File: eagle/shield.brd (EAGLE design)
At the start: 61.9 x 55.9 mm, 14 parts

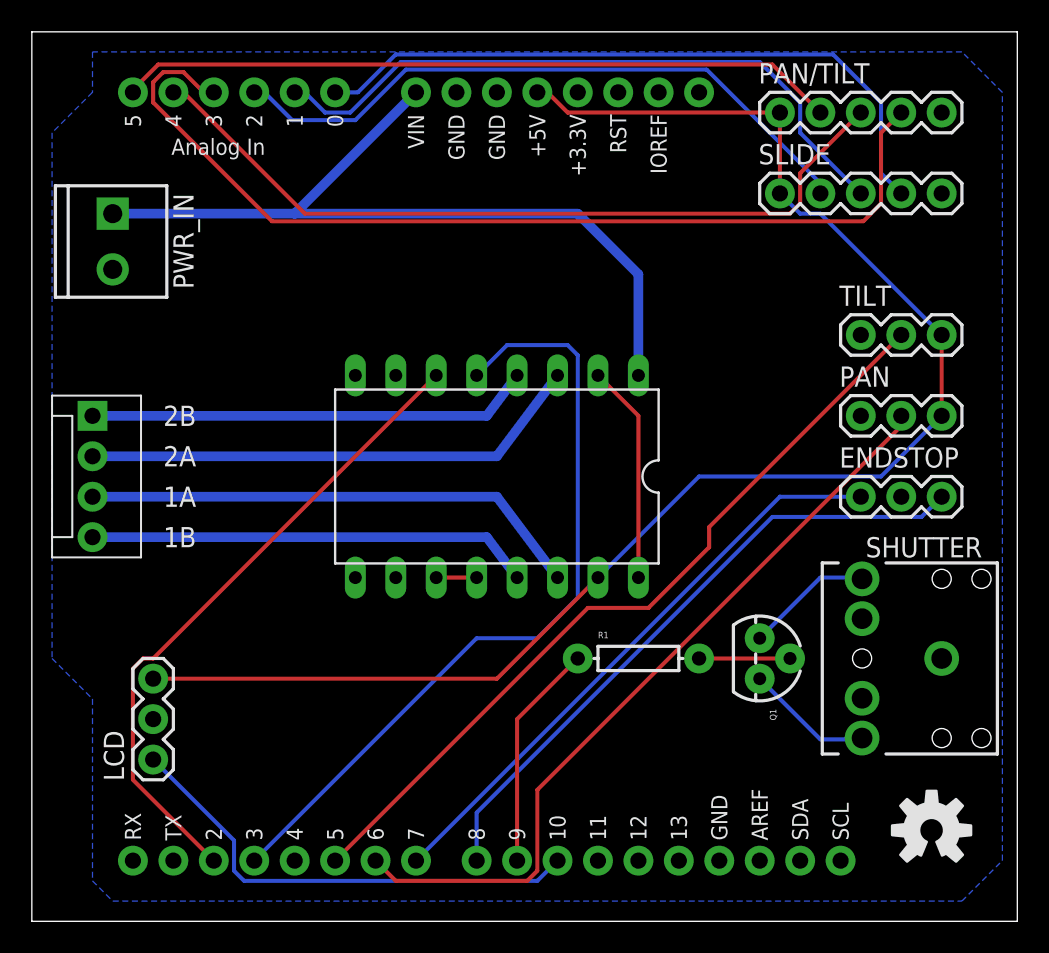
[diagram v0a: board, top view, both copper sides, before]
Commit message: refined board design
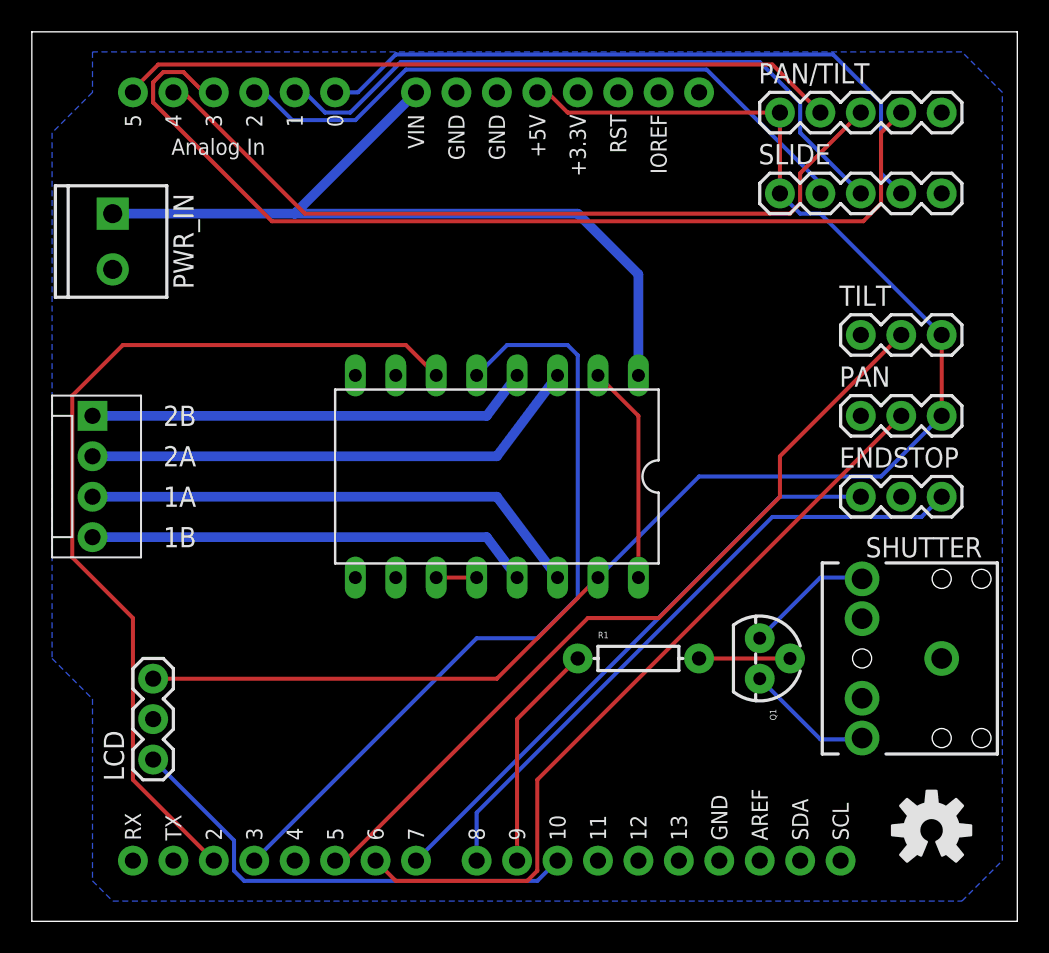
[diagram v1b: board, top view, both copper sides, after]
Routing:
- net N$1: track 40.8 -> 57.9 mm
- net N$18: track 50.0 -> 50.7 mm
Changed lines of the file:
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@@
 <contactref element="MCU" pad="D2"/>
 <contactref element="SOCKET" pad="10"/>
-<wire x1="8.89" y1="39.37" x2="26.67" y2="57.15" width="0.254" layer="1"/>
-<wire x1="8.255" y1="39.37" x2="8.89" y2="39.37" width="0.254" layer="1"/>
-<wire x1="7.62" y1="38.735" x2="8.255" y2="39.37" width="0.254" layer="1"/>
-<wire x1="7.62" y1="31.75" x2="7.62" y2="38.735" width="0.254" layer="1"/>
+<wire x1="7.62" y1="31.75" x2="7.62" y2="41.91" width="0.254" layer="1"/>
 <wire x1="12.7" y1="26.67" x2="7.62" y2="31.75" width="0.254" layer="1"/>
+<wire x1="7.62" y1="41.91" x2="3.81" y2="45.72" width="0.254" layer="1"/>
+<wire x1="3.81" y1="45.72" x2="3.81" y2="55.88" width="0.254" layer="1"/>
+<wire x1="3.81" y1="55.88" x2="6.985" y2="59.055" width="0.254" layer="1"/>
+<wire x1="6.985" y1="59.055" x2="24.765" y2="59.055" width="0.254" layer="1"/>
+<wire x1="24.765" y1="59.055" x2="26.67" y2="57.15" width="0.254" layer="1"/>
 </signal>
 <signal name="N$2">
@@
 <contactref element="PAN" pad="2"/>
 <wire x1="24.13" y1="25.4" x2="22.86" y2="26.67" width="0.254" layer="1"/>
-<wire x1="55.88" y1="53.975" x2="33.02" y2="31.115" width="0.254" layer="1"/>
-<wire x1="55.88" y1="54.61" x2="55.88" y2="53.975" width="0.254" layer="1"/>
 <wire x1="32.385" y1="25.4" x2="24.13" y2="25.4" width="0.254" layer="1"/>
 <wire x1="33.02" y1="26.035" x2="32.385" y2="25.4" width="0.254" layer="1"/>
-<wire x1="33.02" y1="31.115" x2="33.02" y2="26.035" width="0.254" layer="1"/>
+<wire x1="33.02" y1="31.75" x2="33.02" y2="26.035" width="0.254" layer="1"/>
+<wire x1="55.88" y1="54.61" x2="33.02" y2="31.75" width="0.254" layer="1"/>
 </signal>
 <signal name="N$18">
 <contactref element="MCU" pad="D5"/>
 <contactref element="TILT" pad="2"/>
-<wire x1="36.195" y1="42.545" x2="20.32" y2="26.67" width="0.254" layer="1"/>
-<wire x1="55.88" y1="59.69" x2="43.815" y2="47.625" width="0.254" layer="1"/>
-<wire x1="43.815" y1="46.355" x2="43.815" y2="47.625" width="0.254" layer="1"/>
-<wire x1="40.005" y1="42.545" x2="43.815" y2="46.355" width="0.254" layer="1"/>
-<wire x1="36.195" y1="42.545" x2="40.005" y2="42.545" width="0.254" layer="1"/>
+<wire x1="20.32" y1="26.67" x2="20.955" y2="26.67" width="0.254" layer="1"/>
+<wire x1="20.955" y1="26.67" x2="36.195" y2="41.91" width="0.254" layer="1"/>
+<wire x1="36.195" y1="41.91" x2="40.64" y2="41.91" width="0.254" layer="1"/>
+<wire x1="40.64" y1="41.91" x2="48.26" y2="49.53" width="0.254" layer="1"/>
+<wire x1="48.26" y1="49.53" x2="48.26" y2="52.07" width="0.254" layer="1"/>
+<wire x1="48.26" y1="52.07" x2="55.88" y2="59.69" width="0.254" layer="1"/>
 </signal>
 <signal name="N$20">
